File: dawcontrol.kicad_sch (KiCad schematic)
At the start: 30 parts, among them SW1 RotaryEncoder, SW2 RotaryEncoder, U1 STM32L552ZETxQ, U10 ER_OLEDM0.91_1x-I2C, U2 74HC165, U3 STM32G0B1KETx, U4 ALPS_RSA0N11M9A0J, U5 ALPS_RSA0N11M9A0J, U6 TB6612FNG, U7 ER_OLEDM0.91_1x-I2C, U8 ER_OLEDM0.91_1x-I2C, U9 ER_OLEDM0.91_1x-I2C

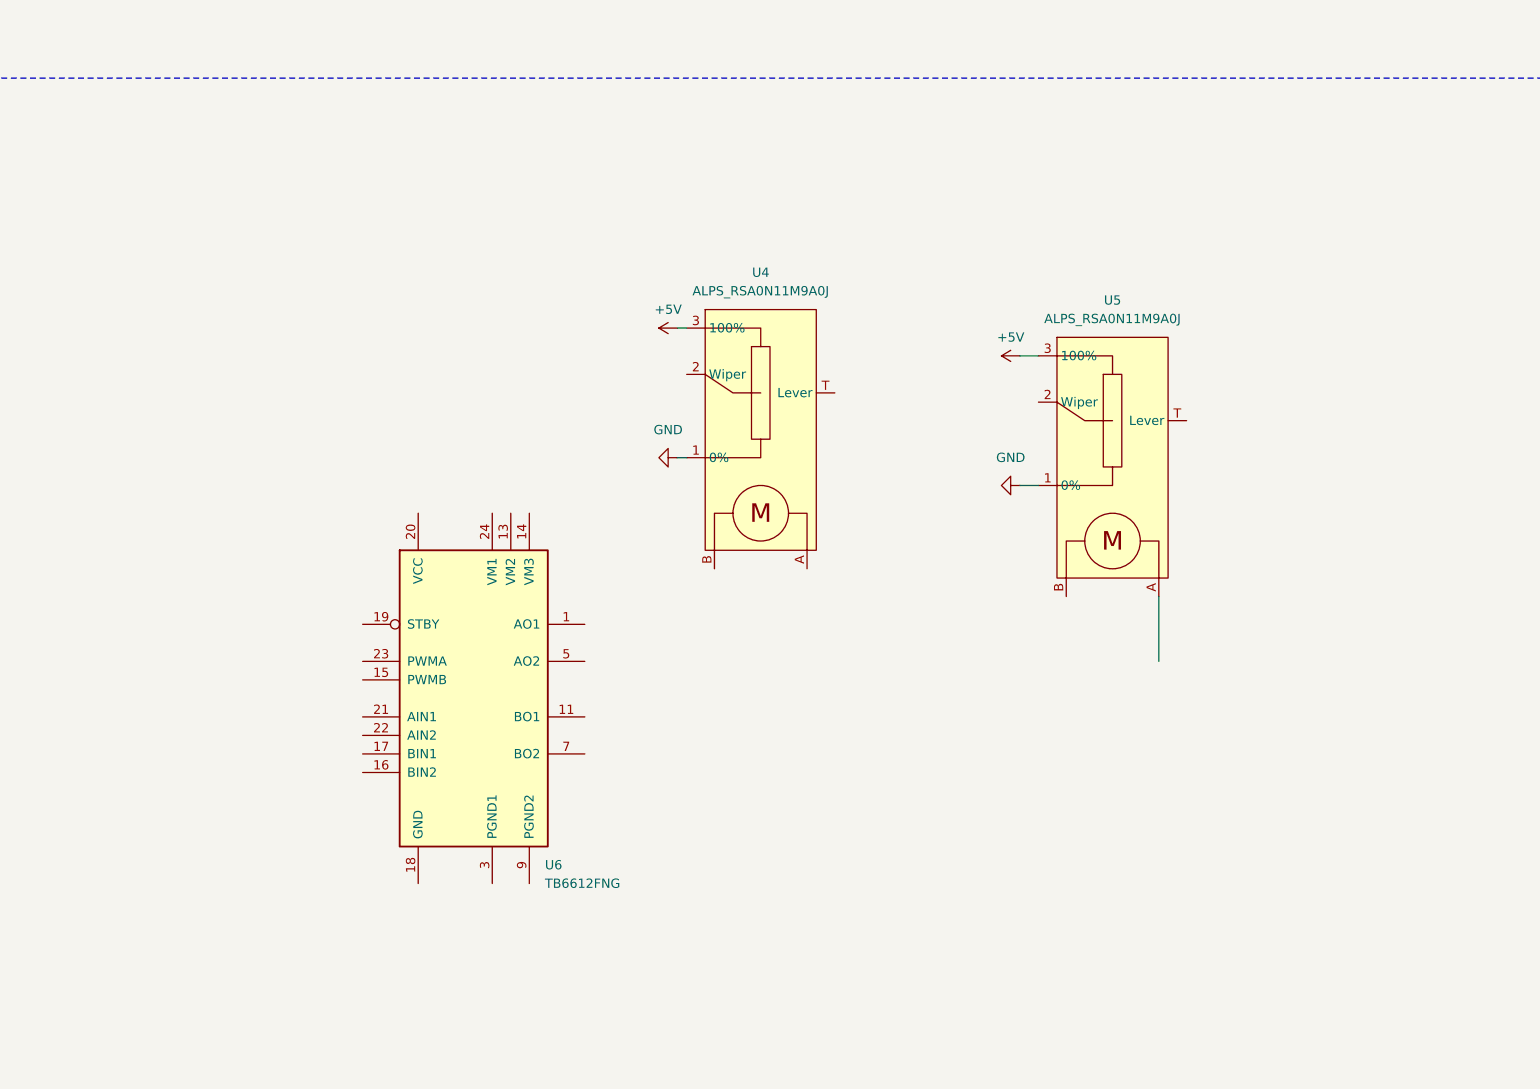
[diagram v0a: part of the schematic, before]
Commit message: Fader section
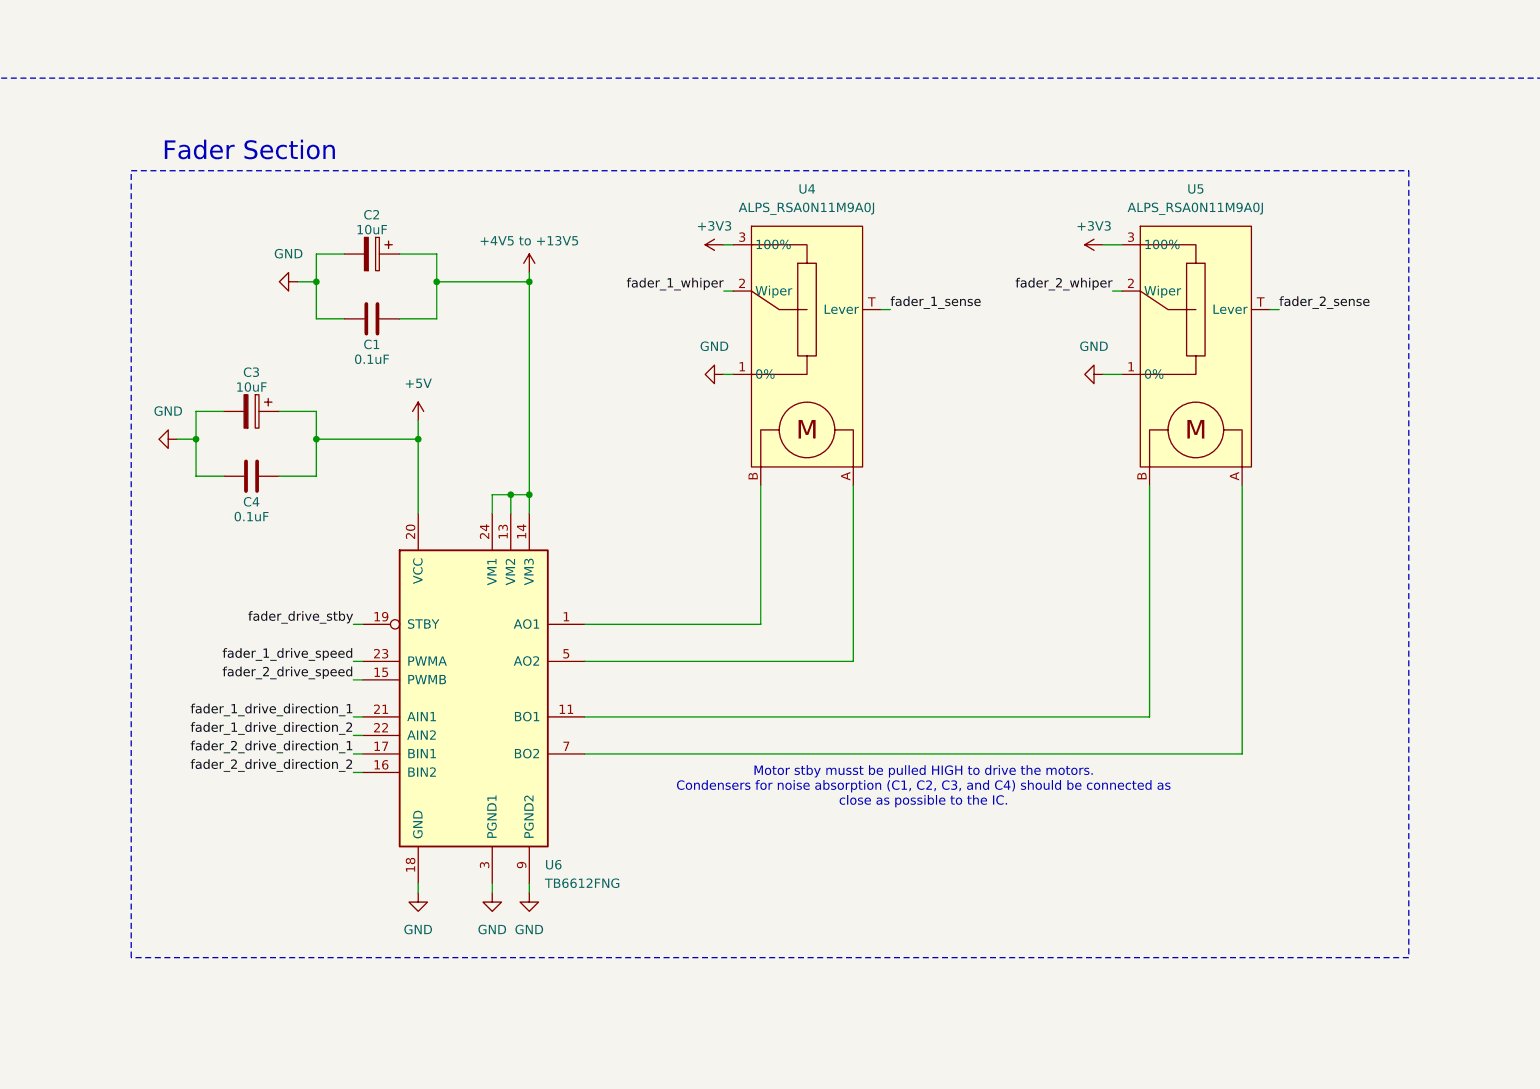
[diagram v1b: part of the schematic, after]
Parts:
- added C1, C4: 0.1uF, symbol Device:C
- added C2, C3: 10uF, symbol Device:C_Polarized
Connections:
- net +5V: now also U6.20 (VCC), C3.1, C4.2; no longer U4.3 (100%), U5.3 (100%)
- net GND: now also U6.10 (PGND2), U6.18 (GND), U6.3 (PGND1), U6.4 (PGND1), U6.9 (PGND2), C1.1, C2.2, C3.2, C4.1
- net fader_1_whiper: now reaches U4.2 (Wiper)
- net at U4.A: now also U6.5 (AO2), U6.6 (AO2)
- net at U4.B: now also U6.1 (AO1), U6.2 (AO1)
- net fader_1_sense: now reaches U4.T (Lever)
- net at U6.11 (BO1), U6.12 (BO1): now also U5.B
- net +4V5 to +13V5: now reaches U6.13 (VM2)
- net +4V5 to +13V5: now also U6.14 (VM3), U6.24 (VM1), C1.2, C2.1
- net fader_2_drive_speed: now reaches U6.15 (PWMB)
- net fader_2_drive_direction_2: now reaches U6.16 (BIN2)
- net fader_2_drive_direction_1: now reaches U6.17 (BIN1)
- net fader_drive_stby: now reaches U6.19 (STBY)
- net fader_1_drive_direction_1: now reaches U6.21 (AIN1)
- net fader_1_drive_direction_2: now reaches U6.22 (AIN2)
- net fader_1_drive_speed: now reaches U6.23 (PWMA)
- net at U6.7 (BO2), U6.8 (BO2): now also U5.A
- net fader_2_whiper: now reaches U5.2 (Wiper)
- net fader_2_sense: now reaches U5.T (Lever)
- new net +3V3: U4.3 (100%), U5.3 (100%)
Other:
- note added: "Fader Section"
- note added: "Motor stby musst be pulled HIGH to drive the motors. Condensers for noise absorption (C1, C2, C3, and C4) should be connected as close as possible to the IC."
- moved on the sheet: U4, U5
